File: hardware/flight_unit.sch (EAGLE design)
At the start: 26 parts, among them IC2 7805T, J1 DCJ0202, J2 CONN_20X2SHROUDED, T1 THERMISTOR-2,5, U1 4MB Flash, U2 4MB Flash, U3 4MB Flash

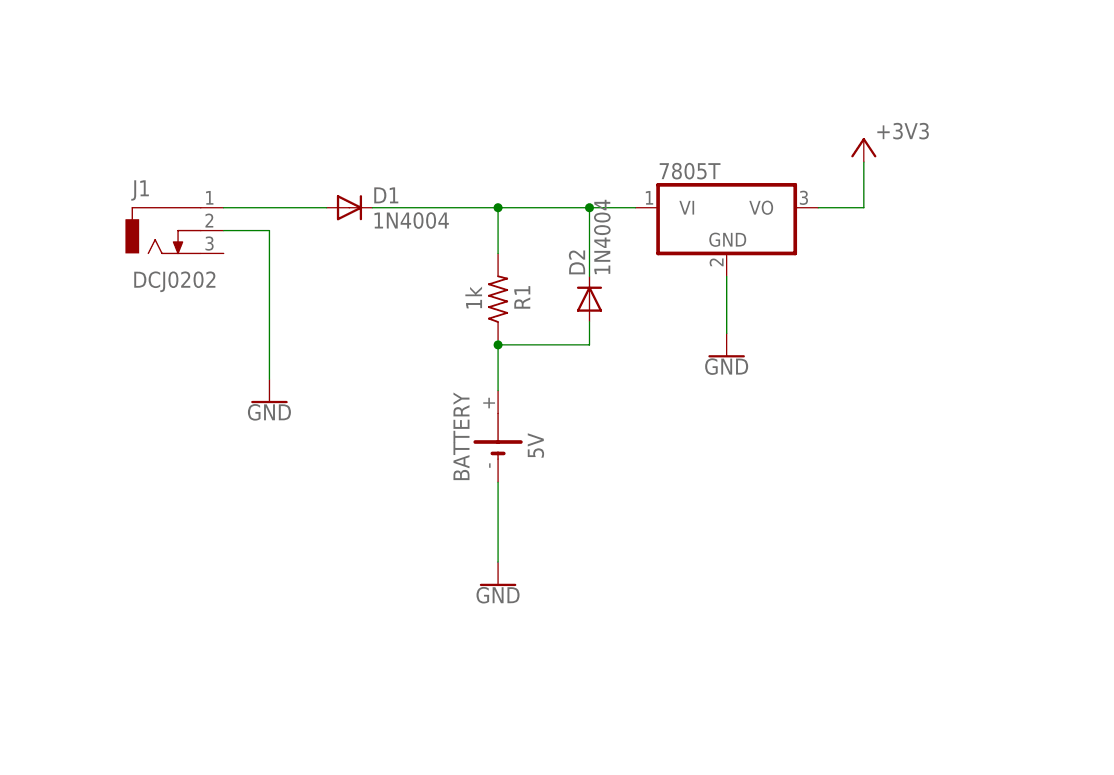
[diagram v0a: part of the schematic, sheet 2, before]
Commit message: Add files via upload
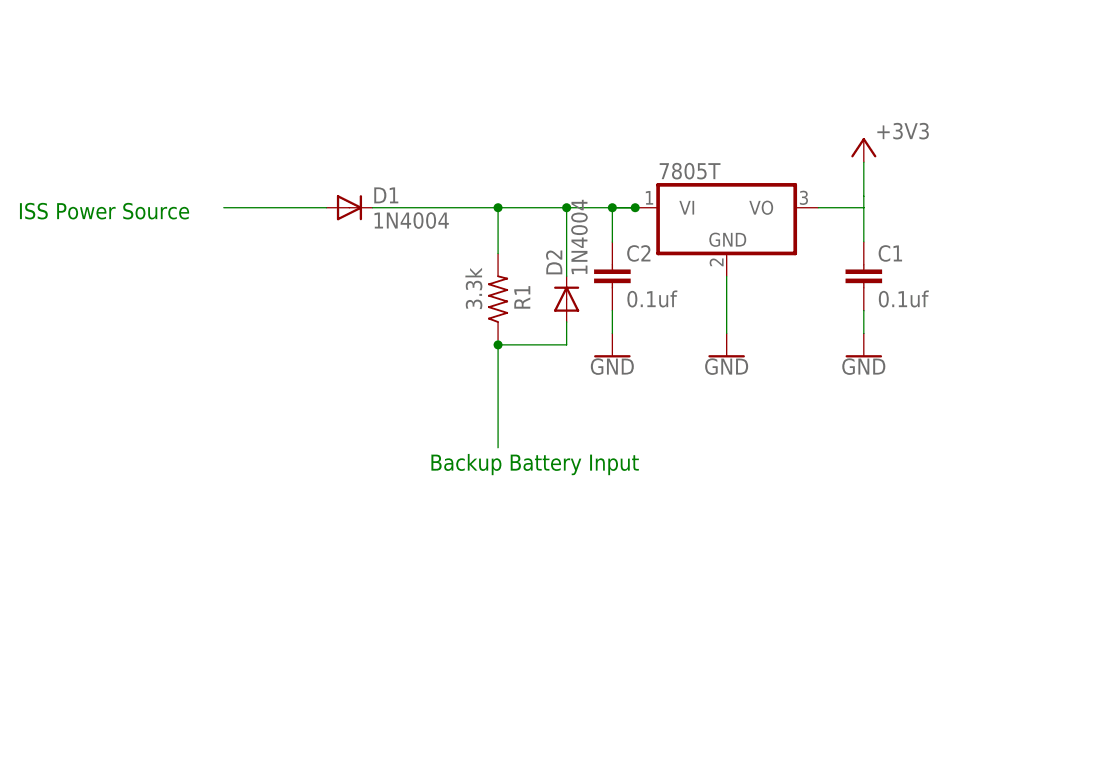
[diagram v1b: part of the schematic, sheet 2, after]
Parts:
- removed BATTERY: 5V, battery:CR-AA
- removed J1: DCJ0202, con-jack:DCJ0202
- added C1, C2: 0.1uf, capacitor-wima:C2,5-3
- R1: value 1k -> 3.3k
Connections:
- net +3V3: now also C1.1
- net GND: now also C1.2, C2.2; no longer BATTERY.-, J1.2
- net N$1: no longer BATTERY.+
- net N$2: now also C2.1
- net N$4: no longer J1.1
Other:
- note added: "Backup Battery Input"
- note added: "ISS Power Source"
- moved on the sheet: D2
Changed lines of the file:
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@@
 <?xml version="1.0" encoding="utf-8"?>
 <!DOCTYPE eagle SYSTEM "eagle.dtd">
-<eagle version="9.5.1">
+<eagle version="9.6.2">
 <drawing>
 <settings>
@@
 <part name="D1" library="diode" library_urn="urn:adsk.eagle:library:210" deviceset="1N4004" device="" package3d_urn="urn:adsk.eagle:package:43336/1"/>
 <part name="D2" library="diode" library_urn="urn:adsk.eagle:library:210" deviceset="1N4004" device="" package3d_urn="urn:adsk.eagle:package:43336/1"/>
-<part name="R1" library="rcl" library_urn="urn:adsk.eagle:library:334" deviceset="R-US_" device="0207/10" package3d_urn="urn:adsk.eagle:package:23491/1" value="1k">
+<part name="R1" library="rcl" library_urn="urn:adsk.eagle:library:334" deviceset="R-US_" device="0207/10" package3d_urn="urn:adsk.eagle:package:23491/1" value="3.3k">
 <attribute name="SPICEPREFIX" value="1000 Ohm"/>
 </part>
-<part name="BATTERY" library="battery" library_urn="urn:adsk.eagle:library:109" deviceset="CR-AA" device="" package3d_urn="urn:adsk.eagle:package:4582/1" value="5V">
-<attribute name="BATTERY" value="5 V"/>
-</part>
-<part name="J1" library="con-jack" library_urn="urn:adsk.eagle:library:154" deviceset="DCJ0202" device="" package3d_urn="urn:adsk.eagle:package:7491/1"/>
 <part name="IC2" library="linear" library_urn="urn:adsk.eagle:library:262" deviceset="78*" device="T" package3d_urn="urn:adsk.eagle:package:16414/1" technology="05"/>
 <part name="+3V1" library="supply1" deviceset="+3V3" device=""/>
@@
 <part name="J2" library="SparkFun-Connectors" library_urn="urn:adsk.eagle:library:513" deviceset="CONN_20X2" device="SHROUDED" package3d_urn="urn:adsk.eagle:package:38279/1"/>
 <part name="GND" library="SparkFun-PowerSymbols" library_urn="urn:adsk.eagle:library:530" deviceset="GND" device=""/>
-<part name="GND1" library="SparkFun-PowerSymbols" library_urn="urn:adsk.eagle:library:530" deviceset="GND" device=""/>
-<part name="GND2" library="SparkFun-PowerSymbols" library_urn="urn:adsk.eagle:library:530" deviceset="GND" device=""/>
 <part name="GND3" library="SparkFun-PowerSymbols" library_urn="urn:adsk.eagle:library:530" deviceset="GND" device=""/>
 <part name="U$1" library="TEENSY 4.0" deviceset="TEENSY_4.0" device=""/>
@@
 <part name="JP1" library="adafruit" deviceset="PINHD-1X6" device="B"/>
 <part name="U$8" library="microbuilder" deviceset="GND" device=""/>
+<part name="C1" library="capacitor-wima" library_urn="urn:adsk.eagle:library:116" deviceset="C" device="2,5-3" package3d_urn="urn:adsk.eagle:package:5436/1" value="0.1uf"/>
+<part name="GND1" library="SparkFun-PowerSymbols" library_urn="urn:adsk.eagle:library:530" deviceset="GND" device=""/>
+<part name="C2" library="capacitor-wima" library_urn="urn:adsk.eagle:library:116" deviceset="C" device="2,5-3" package3d_urn="urn:adsk.eagle:package:5436/1" value="0.1uf"/>
+<part name="GND2" library="SparkFun-PowerSymbols" library_urn="urn:adsk.eagle:library:530" deviceset="GND" device=""/>
 </parts>
 <sheets>
@@
 </text>
 <text x="82.55" y="161.29" size="5.08" layer="97">Power Regulation and Supply</text>
+<text x="68.58" y="109.22" size="1.778" layer="91">ISS Power Source</text>
+<text x="114.3" y="81.28" size="1.778" layer="91">Backup Battery Input </text>
 </plain>
 <instances>
@@
 <attribute name="VALUE" x="107.95" y="108.1786" size="1.778" layer="96"/>
 </instance>
-<instance part="D2" gate="1" x="132.08" y="100.33" smashed="yes" rot="R90">
-<attribute name="NAME" x="131.5974" y="102.87" size="1.778" layer="95" rot="R90"/>
-<attribute name="VALUE" x="134.3914" y="102.87" size="1.778" layer="96" rot="R90"/>
+<instance part="D2" gate="1" x="129.54" y="100.33" smashed="yes" rot="R90">
+<attribute name="NAME" x="129.0574" y="102.87" size="1.778" layer="95" rot="R90"/>
+<attribute name="VALUE" x="131.8514" y="102.87" size="1.778" layer="96" rot="R90"/>
 </instance>
 <instance part="R1" gate="G$1" x="121.92" y="100.33" smashed="yes" rot="R90">
@@
 <attribute name="SPICEPREFIX" x="121.92" y="100.33" size="1.778" layer="96" rot="R90" display="off"/>
 </instance>
-<instance part="BATTERY" gate="1" x="121.92" y="85.09" smashed="yes" rot="R90">
-<attribute name="NAME" x="118.745" y="80.01" size="1.778" layer="95" rot="R90"/>
-<attribute name="VALUE" x="127" y="82.55" size="1.778" layer="96" rot="R90"/>
-<attribute name="BATTERY" x="121.92" y="85.09" size="1.778" layer="96" rot="R90" display="off"/>
-</instance>
-<instance part="J1" gate="G$1" x="83.82" y="107.95" smashed="yes">
-<attribute name="NAME" x="81.28" y="111.76" size="1.778" layer="95"/>
-<attribute name="VALUE" x="81.28" y="101.6" size="1.778" layer="96"/>
-</instance>
 <instance part="IC2" gate="A1" x="147.32" y="110.49" smashed="yes">
 <attribute name="VALUE" x="139.7" y="113.665" size="1.778" layer="96"/>
@@
 <attribute name="VALUE" x="163.83" y="118.11" size="1.778" layer="96"/>
 </instance>
-<instance part="GND1" gate="1" x="96.52" y="88.9" smashed="yes">
-<attribute name="VALUE" x="96.52" y="88.646" size="1.778" layer="96" align="top-center"/>
-</instance>
-<instance part="GND2" gate="1" x="121.92" y="68.58" smashed="yes">
-<attribute name="VALUE" x="121.92" y="68.326" size="1.778" layer="96" align="top-center"/>
-</instance>
 <instance part="GND3" gate="1" x="147.32" y="93.98" smashed="yes">
 <attribute name="VALUE" x="147.32" y="93.726" size="1.778" layer="96" align="top-center"/>
+</instance>
+<instance part="C1" gate="G$1" x="162.56" y="104.14" smashed="yes">
+<attribute name="NAME" x="164.084" y="104.521" size="1.778" layer="95"/>
+<attribute name="VALUE" x="164.084" y="99.441" size="1.778" layer="96"/>
+</instance>
+<instance part="GND1" gate="1" x="162.56" y="93.98" smashed="yes">
+<attribute name="VALUE" x="162.56" y="93.726" size="1.778" layer="96" align="top-center"/>
+</instance>
+<instance part="C2" gate="G$1" x="134.62" y="104.14" smashed="yes">
+<attribute name="NAME" x="136.144" y="104.521" size="1.778" layer="95"/>
+<attribute name="VALUE" x="136.144" y="99.441" size="1.778" layer="96"/>
+</instance>
+<instance part="GND2" gate="1" x="134.62" y="93.98" smashed="yes">
+<attribute name="VALUE" x="134.62" y="93.726" size="1.778" layer="96" align="top-center"/>
 </instance>
 </instances>
@@
 <net name="N$1" class="0">
 <segment>
-<pinref part="BATTERY" gate="1" pin="+"/>
 <pinref part="R1" gate="G$1" pin="1"/>
-<wire x1="121.92" y1="90.17" x2="121.92" y2="95.25" width="0.1524" layer="91"/>
+<pinref part="D2" gate="1" pin="A"/>
+<wire x1="121.92" y1="95.25" x2="129.54" y2="95.25" width="0.1524" layer="91"/>
+<wire x1="129.54" y1="95.25" x2="129.54" y2="97.79" width="0.1524" layer="91"/>
+<wire x1="121.92" y1="95.25" x2="121.92" y2="83.82" width="0.1524" layer="91"/>
 <junction x="121.92" y="95.25"/>
-<pinref part="D2" gate="1" pin="A"/>
-<wire x1="121.92" y1="95.25" x2="132.08" y2="95.25" width="0.1524" layer="91"/>
-<wire x1="132.08" y1="95.25" x2="132.08" y2="97.79" width="0.1524" layer="91"/>
 </segment>
 </net>
@@
 <junction x="121.92" y="110.49"/>
 <pinref part="D2" gate="1" pin="C"/>
-<wire x1="132.08" y1="110.49" x2="121.92" y2="110.49" width="0.1524" layer="91"/>
-<wire x1="132.08" y1="102.87" x2="132.08" y2="110.49" width="0.1524" layer="91"/>
-<wire x1="132.08" y1="110.49" x2="137.16" y2="110.49" width="0.1524" layer="91"/>
-<junction x="132.08" y="110.49"/>
+<wire x1="129.54" y1="110.49" x2="121.92" y2="110.49" width="0.1524" layer="91"/>
+<wire x1="129.54" y1="102.87" x2="129.54" y2="110.49" width="0.1524" layer="91"/>
+<wire x1="129.54" y1="110.49" x2="137.16" y2="110.49" width="0.1524" layer="91"/>
+<junction x="129.54" y="110.49"/>
 <pinref part="IC2" gate="A1" pin="VI"/>
+<pinref part="C2" gate="G$1" pin="1"/>
+<wire x1="134.62" y1="106.68" x2="134.62" y2="110.49" width="0.1524" layer="91"/>
+<wire x1="134.62" y1="110.49" x2="137.16" y2="110.49" width="0.1524" layer="91"/>
+<junction x="137.16" y="110.49"/>
 </segment>
 </net>
 <net name="N$4" class="0">
 <segment>
-<pinref part="J1" gate="G$1" pin="1"/>
 <pinref part="D1" gate="1" pin="A"/>
 <wire x1="91.44" y1="110.49" x2="102.87" y2="110.49" width="0.1524" layer="91"/>
@@
 <pinref part="IC2" gate="A1" pin="VO"/>
 <pinref part="+3V1" gate="G$1" pin="+3V3"/>
-<wire x1="162.56" y1="115.57" x2="162.56" y2="110.49" width="0.1524" layer="91"/>
+<wire x1="162.56" y1="115.57" x2="162.56" y2="111.76" width="0.1524" layer="91"/>
+<pinref part="C1" gate="G$1" pin="1"/>
+<wire x1="162.56" y1="111.76" x2="162.56" y2="110.49" width="0.1524" layer="91"/>
+<wire x1="162.56" y1="106.68" x2="162.56" y2="110.49" width="0.1524" layer="91"/>
 </segment>
 </net>
 <net name="GND" class="0">
-<segment>
-<pinref part="J1" gate="G$1" pin="2"/>
-<pinref part="GND1" gate="1" pin="GND"/>
-<wire x1="91.44" y1="107.95" x2="96.52" y2="107.95" width="0.1524" layer="91"/>
-<wire x1="96.52" y1="107.95" x2="96.52" y2="91.44" width="0.1524" layer="91"/>
-</segment>
-<segment>
-<pinref part="BATTERY" gate="1" pin="-"/>
-<pinref part="GND2" gate="1" pin="GND"/>
-<wire x1="121.92" y1="80.01" x2="121.92" y2="71.12" width="0.1524" layer="91"/>
-</segment>
 <segment>
 <pinref part="IC2" gate="A1" pin="GND"/>
@@
 <wire x1="147.32" y1="102.87" x2="147.32" y2="96.52" width="0.1524" layer="91"/>
 </segment>
-</net>
+<segment>
+<pinref part="C1" gate="G$1" pin="2"/>
+<pinref part="GND1" gate="1" pin="GND"/>
+<wire x1="162.56" y1="99.06" x2="162.56" y2="96.52" width="0.1524" layer="91"/>
+</segment>
+<segment>
+<pinref part="C2" gate="G$1" pin="2"/>
+<pinref part="GND2" gate="1" pin="GND"/>
+<wire x1="134.62" y1="99.06" x2="134.62" y2="96.52" width="0.1524" layer="91"/>
+</segment>
+</net>
+<net name="N$9" class="0">
+<segment>
+<junction x="134.62" y="110.49"/>
+</segment>
+</net>
